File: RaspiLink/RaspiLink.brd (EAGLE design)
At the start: 65 x 55.9 mm, 20 parts, among them Q1 MOSFET-NCHANNELBSS123LT1G, Q2 MOSFET-NCHANNELBSS123LT1G, X1 SSW-120-02-S-D, X2 SSW-120-02-S-S, X3 SSW-120-02-S-S, X4 SSW-108-02-S-D

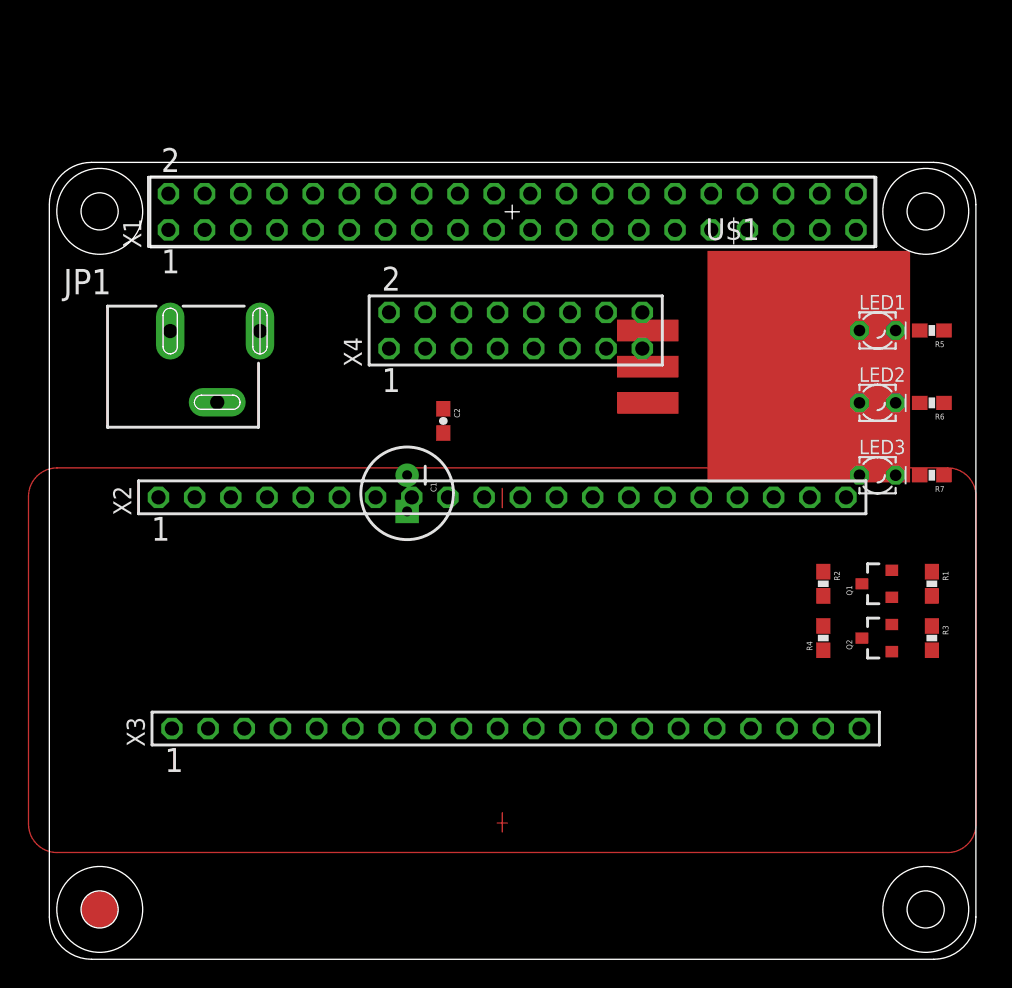
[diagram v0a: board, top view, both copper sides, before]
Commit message: joystick for crane
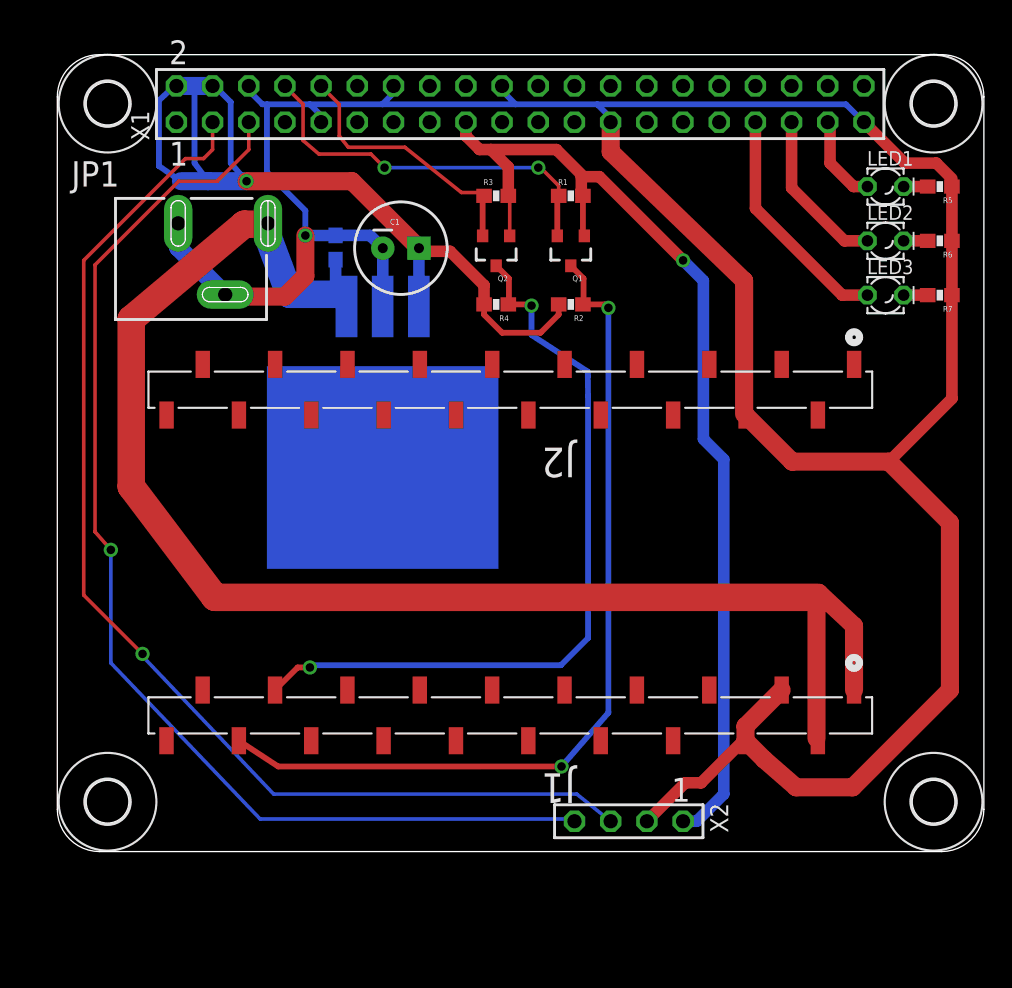
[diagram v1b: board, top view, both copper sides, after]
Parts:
- removed X3: SSW-120-02-S-S, con-samtec:SSW-120-02-S-S
- removed X4: SSW-108-02-S-D, con-samtec:SSW-108-02-S-D
- added J1, J2: SSM-120-S-SV, SAMTEC-FLE-Mxx-Sxx_By_element14_Batch_1:SAMTEC_SSM-120-S-SV
- added U$2, U$3, U$4, U$5: (no value), holes:3,0
- X2: value SSW-120-02-S-S -> SSW-104-02-S-S; device con-samtec:SSW-120-02-S-S -> con-samtec:SSW-104-02-S-S
- moved R3 43.6 mm to (27.8, 50.1), turned to 0 degrees
- moved Q2 38.2 mm to (27.8, 46.3), turned to 180 degrees
- moved R1 37.2 mm to (33.1, 50.1), turned to 0 degrees
- moved R4 32.8 mm to (27.8, 42.5), turned to 180 degrees
- moved Q1 31.8 mm to (33.1, 46.3), turned to 180 degrees
- moved R2 26.4 mm to (33.1, 42.5), turned to 180 degrees
- moved U$1 24.6 mm to (19.9, 36.4), flipped to the bottom, turned to 270 degrees
- moved X2 24.4 mm to (37.1, 6.19), turned to 180 degrees
- moved C1 17.2 mm to (21.2, 46.4), turned to 0 degrees
- moved C2 14.3 mm to (16.6, 46.5), flipped to the bottom, turned to 90 degrees
- moved LED3 12.7 mm to (55.2, 43.1)
- moved R7 12.7 mm to (59.0, 43.1)
- moved LED2 11.4 mm to (55.2, 46.9)
- moved R6 11.4 mm to (59.0, 46.9)
- moved LED1 10.1 mm to (55.2, 50.7)
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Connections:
- removed net CM_RXD_1: X2.17, X4.4
- removed net CM_RXD_2: X2.10, X4.15
- removed net CM_TXD_1: X2.16, X4.2
- removed net CM_TXD_2: X2.9, X4.13
- removed net GPIO10_MOSI: X1.19, X4.12
- removed net GPIO11_CLK: X1.23, X4.14
- removed net GPIO17: X1.11
- removed net GPIO18_PWM: X1.12, X4.11
- removed net GPIO22: X1.15
- removed net GPIO23: LED3.A, X1.16
- removed net GPIO24: LED2.A, X1.18
- removed net GPIO25: LED1.A, X1.22
- removed net GPIO27: X1.13
- removed net GPIO4: X1.7
- removed net GPIO7_CE1: X1.26, X4.6
- removed net GPIO8_CE0: X1.24, X4.8
- removed net GPIO9_MISO: X1.21, X4.10
- new net GPIO13: LED3.A, X1.33
- new net GPIO19: LED2.A, X1.35
- new net GPIO26: LED1.A, X1.37
- net +3.3V: now also X2.1; no longer X1.1, X4.1
- net +5V: no longer X4.3
- net CM_RX: now also J1.18; no longer X3.18
- net CM_TX: now also J1.17; no longer X3.17
- net GND: now also J1.3, J1.4, J2.4, X1.39, X2.2; no longer X2.4, X3.3, X3.4, X4.16, X4.5
- net I2C_SCL: now also X2.4; no longer X4.9
- net I2C_SDA: now also X2.3; no longer X4.7
- net VCC: now also J1.1, J1.2; no longer X3.1, X3.2
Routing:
- net GND: track 0.00 -> 177.7 mm, vias 0 -> 1
- net VCC: track 0.00 -> 108.5 mm, vias 0 -> 1
- net I2C_SCL: track 0.00 -> 81.7 mm, vias 0 -> 1
- net I2C_SDA: track 0.00 -> 81.4 mm, vias 0 -> 1
- net +3.3V: track 0.00 -> 73.1 mm, vias 0 -> 1
- net N$6: track 65.3 -> 0.00 mm
- net +5V: track 0.00 -> 63.6 mm, vias 0 -> 1
- net N$4: track 62.5 -> 0.00 mm
- net CM_RX: track 0.00 -> 61.6 mm, vias 0 -> 2
- net CM_TX: track 0.00 -> 53.7 mm, vias 0 -> 2
- net PI_TX: track 0.00 -> 27.1 mm, vias 0 -> 2
- net N$5: track 25.8 -> 0.00 mm
- net N$2: track 23.0 -> 0.00 mm
- net N$1: track 2.82 -> 24.5 mm
- net PI_RX: track 0.00 -> 18.6 mm
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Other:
- outline, holes or cut-outs redrawn
